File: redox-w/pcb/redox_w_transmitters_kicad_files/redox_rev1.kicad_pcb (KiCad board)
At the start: 2 copper layers, 162.2 x 126.5 mm, 83 parts, among them K0 KEYSW, K1 KEYSW, K10 KEYSW, K11 KEYSW, K12 KEYSW, K13 KEYSW, K14 KEYSW, K15 KEYSW, K16 KEYSW, K2 KEYSW, K20 KEYSW, K21 KEYSW, K22 KEYSW, K23 KEYSW, K24 KEYSW, K25 KEYSW, K26 KEYSW, K3 KEYSW, K30 KEYSW, K31 KEYSW, K32 KEYSW, K33 KEYSW, K34 KEYSW, K35 KEYSW, K36 KEYSW, K4 KEYSW, K40 KEYSW, K41 KEYSW, K42 KEYSW, K43 KEYSW, K44 KEYSW, K45 KEYSW, K46 KEYSW, K5 KEYSW, K6 KEYSW

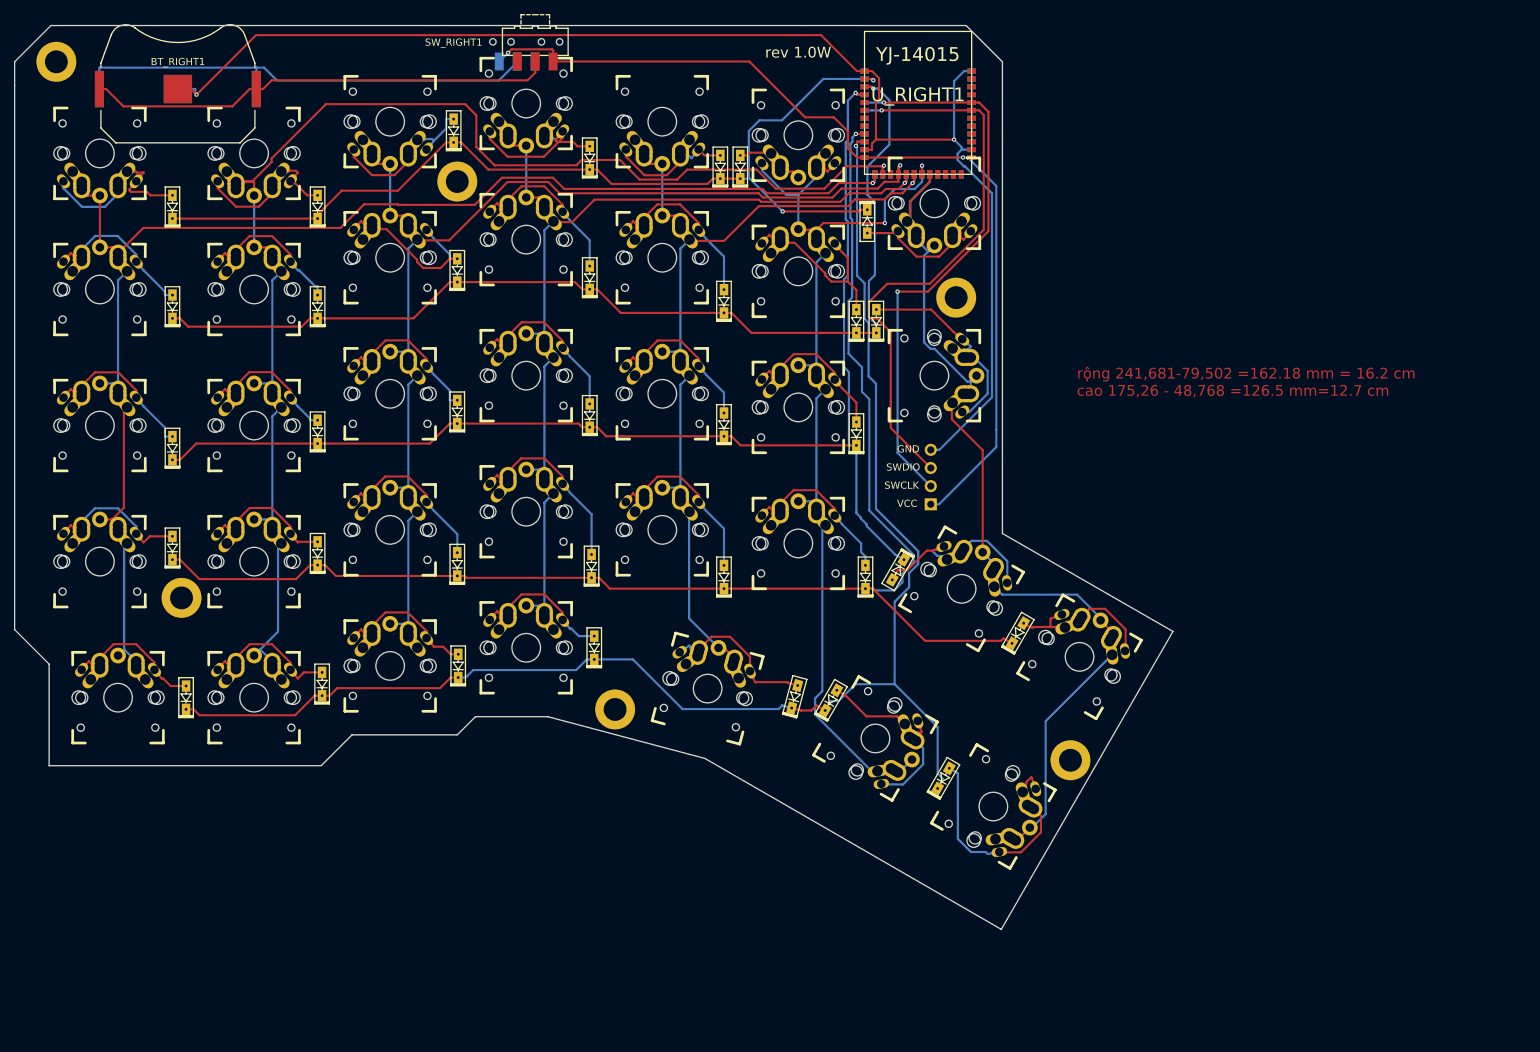
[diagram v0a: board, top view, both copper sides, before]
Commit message: cap nhat 12:00 18/03/2021
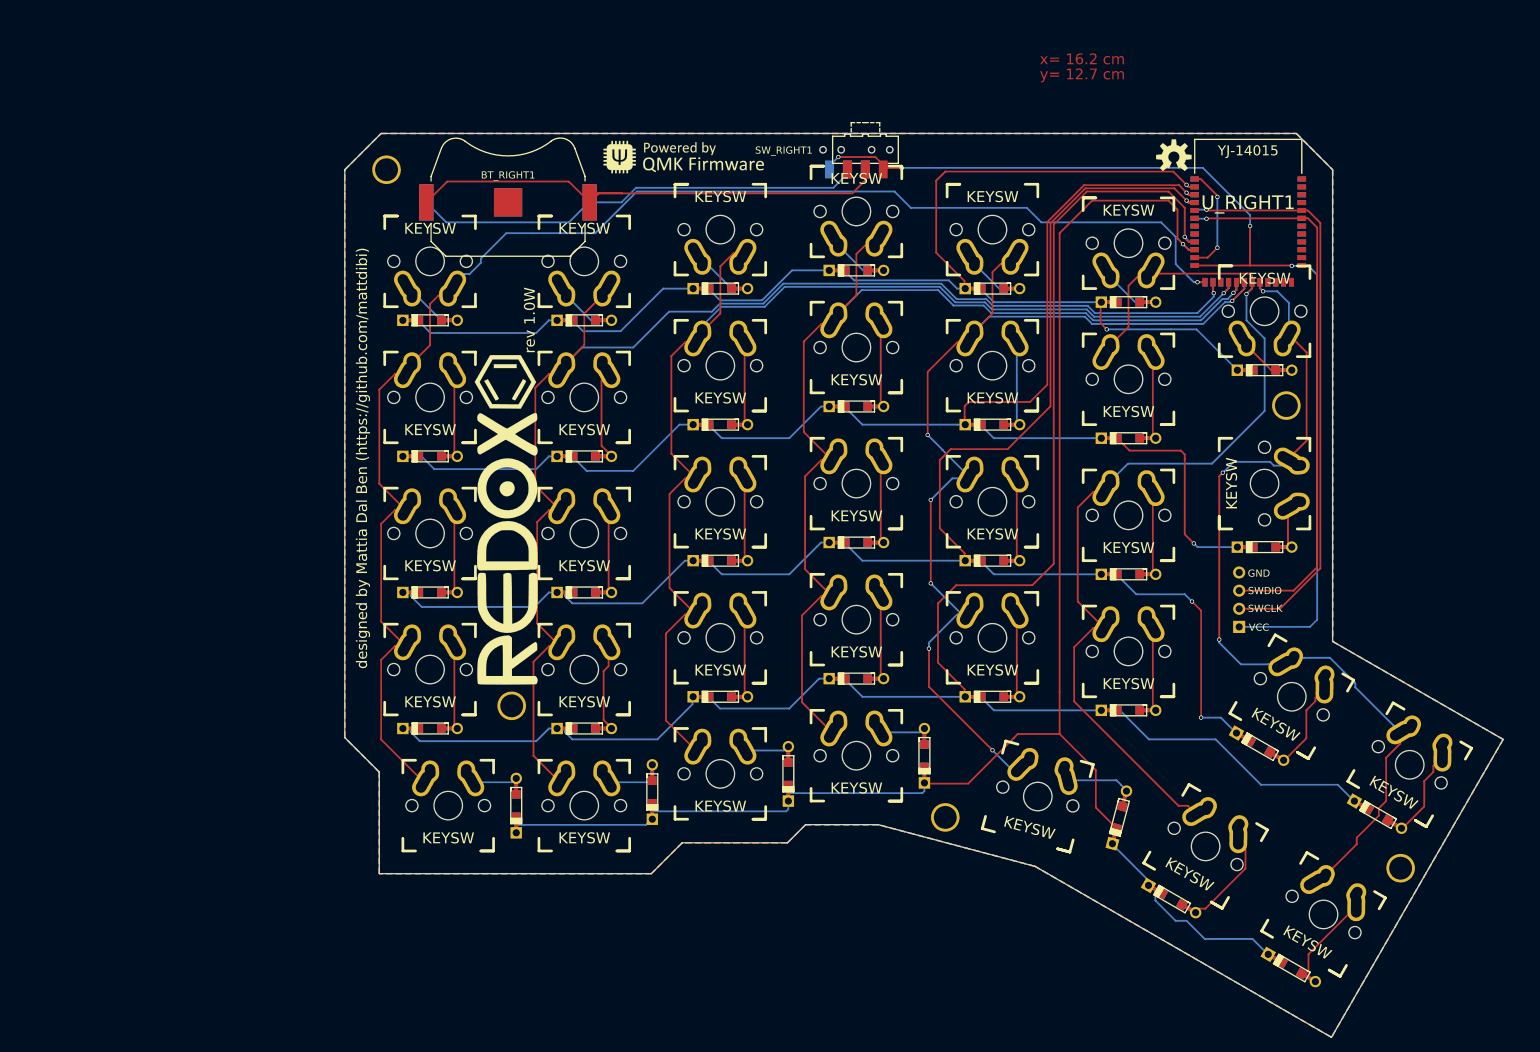
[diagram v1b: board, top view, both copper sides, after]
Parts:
- removed H1, H2, H3, H4, H5, H6: , fruitkey:Hole_M3
- added ?: , Sparkfun-Aesthetics:OSHW-LOGO-M, B.Cu at (195.6, 52.1)
- added ?: , Sparkfun-Aesthetics:OSHW-LOGO-M, F.Cu at (195.6, 52.1)
- added G***: LOGO, myparts:qmk-badge, B.Cu at (127.0, 52.1)
- added G***: LOGO, myparts:redox-logo, F.Cu at (102.2, 102.9)
- added G***: LOGO, myparts:redox-logo, B.Cu at (102.2, 102.2)
- added G***: LOGO, myparts:qmk-badge, F.Cu at (127.0, 52.1)
- added HOLE_M3: VAL**, keyboard_parts:HOLE_M3, F.Cu at (163.6, 144.5)
- added HOLE_M3: VAL**, keyboard_parts:HOLE_M3, F.Cu at (227.3, 151.6)
- added HOLE_M3: VAL**, keyboard_parts:HOLE_M3, F.Cu at (85.3, 53.8)
- added HOLE_M3: VAL**, keyboard_parts:HOLE_M3, F.Cu at (211.3, 86.9)
- added HOLE_M3: VAL**, keyboard_parts:HOLE_M3, F.Cu at (102.9, 128.9)
- BT_LEFT1, BT_RIGHT1: footprint Battery:BatteryHolder_Keystone_3034_1x20mm -> redox_w_footprints:BatteryHolder_Keystone_3034_1x20mm
- D0, D1, D10, D11, D12, D13, D14, D15, D16, D2, D20, D21, D22, D23, D24, D25, D26, D3, D30, D31, D32, D33, D34, D35, D36, D4, D40, D41, D42, D43, D44, D45, D46, D5, D6: footprint fruitkey:Diode_smd -> redox_w_footprints:Diode-dual
- J_PROG_PORT1: footprint Connector_PinHeader_2.54mm:PinHeader_1x04_P2.54mm_Horizontal -> Connector_PinHeader_2.54mm:PinHeader_1x04_P2.54mm_Vertical
- K0, K1, K10, K11, K12, K13, K14, K15, K16, K2, K20, K21, K22, K23, K24, K25, K26, K3, K30, K31, K32, K33, K34, K35, K36, K4, K40, K41, K42, K43, K44, K45, K46, K5, K6: footprint Switch_2_mat:1u -> redox_w_footprints:Mx_Alps_100-dualside
- moved D16 62.9 mm to (208.3, 106.7), turned to 180 degrees
- moved D6 59.4 mm to (208.3, 81.9), turned to 180 degrees
- moved D5 57.6 mm to (189.2, 72.4), turned to 180 degrees
- moved D36 56.5 mm to (224.2, 144.1), turned to 150 degrees
- moved D26 56.4 mm to (207.6, 134.6), turned to 150 degrees
- moved D46 55.5 mm to (212.1, 165.6), turned to 150 degrees
- moved D45 55.3 mm to (195.3, 156.0), turned to 150 degrees
- moved BT_LEFT1 48.9 mm to (102.4, 58.4)
- moved BT_RIGHT1 48.9 mm to (102.4, 58.4)
- moved K42 48.6 mm to (132.1, 138.4)
- moved U_LEFT1 48.6 mm to (206.0, 69.6)
- moved U_RIGHT1 48.6 mm to (206.0, 69.6)
- moved D41 48.6 mm to (122.6, 141.0), turned to 270 degrees
- moved K12 48.6 mm to (132.1, 81.3)
- moved K14 48.6 mm to (170.2, 81.3)
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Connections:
- K5 pad 1: Net-(D5-Pad2) -> col5
- K5 pad 2: col5 -> Net-(D5-Pad2)
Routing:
- net GND: track 193.2 -> 15.2 mm
- net row3: track 200.2 -> 250.7 mm
- net row1: track 145.4 -> 195.1 mm, vias 1 -> 2
- net row2: track 172.4 -> 221.4 mm, vias 1 -> 3
- net row0: track 135.4 -> 181.1 mm
- net Net-(D16-Pad2): track 31.6 -> 5.75 mm
- net Net-(D46-Pad2): track 36.2 -> 12.7 mm
- net Net-(D3-Pad2): track 27.6 -> 5.53 mm
- net Net-(D0-Pad2): track 26.0 -> 7.05 mm
- net VCC: track 130.1 -> 148.2 mm, vias 2 -> 4
- net Net-(D33-Pad2): track 29.5 -> 11.7 mm
- net Net-(D41-Pad2): track 23.3 -> 6.21 mm
- net Net-(D15-Pad2): track 28.8 -> 11.7 mm
- net Net-(D1-Pad2): track 22.6 -> 5.53 mm
- net Net-(D40-Pad2): track 23.4 -> 6.38 mm
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- added copper zone on B.Cu, net (none)
- added copper zone on F.Cu, net (none)
- added copper zone on B.Cu, net GND
- added copper zone on F.Cu, net GND
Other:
- net class Default: clearance 0.3 -> 0.2; trace_width 0.3 -> 0.25
- rule trace_clearance: 0.3 -> 0.2
- board text added: "designed by Mattia Dal Ben (https://github.com/mattdibi)"
- board text added: "x= 16.2 cm"
- board text added: "y= 12.7 cm"
- board text removed: "rộng 241,681-79,502 =162.18 mm = 16.2 cm cao 175,26 - 48,768 =126.5 mm=12.7 cm"
